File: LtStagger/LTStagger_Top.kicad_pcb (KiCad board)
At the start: 2 copper layers, 155 x 112 mm, 9 parts

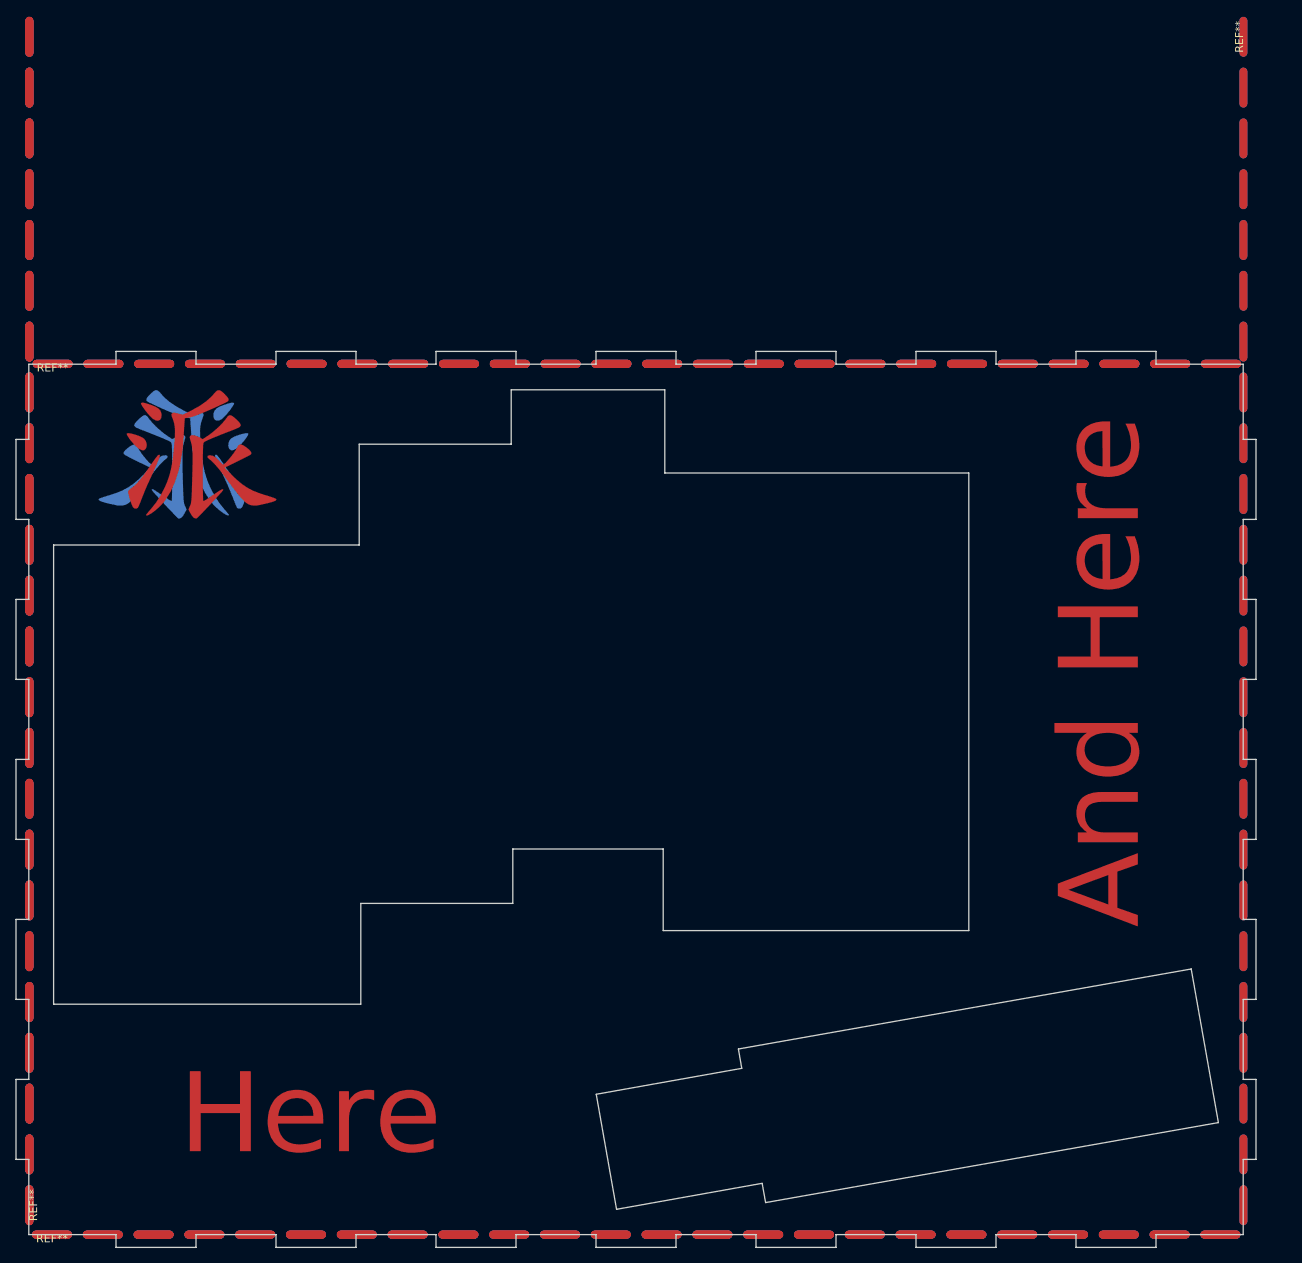
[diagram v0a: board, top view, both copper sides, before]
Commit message: about to give an angle and dog bones
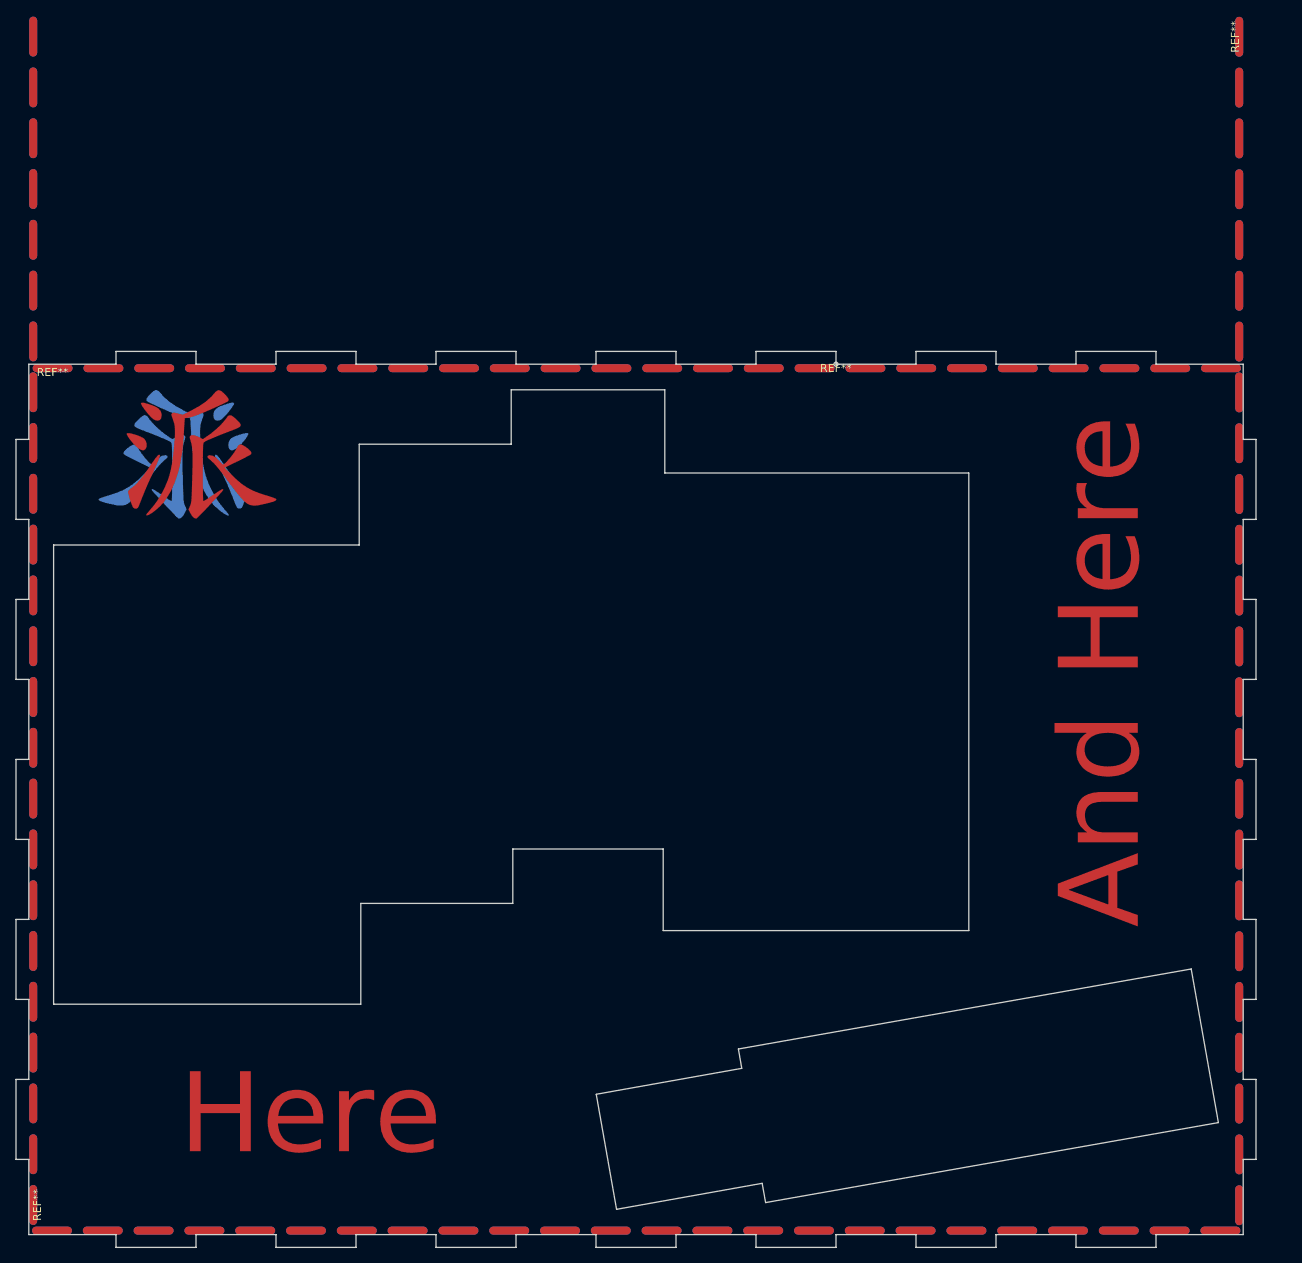
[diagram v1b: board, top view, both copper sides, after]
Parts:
- removed the REF** at (64.0, 147.5)
- removed the REF** at (66.8, 151.2)
- removed the REF** at (66.9, 42.4)
- added REF**: 0.5mmHole, Digi:0.5mmHole, F.Cu at (164.8, 42.4)
- moved REF** 0.55 mm to (66.9, 42.9)
- moved REF** 0.53 mm to (215.2, 1.48)
- moved REF** 0.50 mm to (66.8, 150.7)
- moved REF** 0.48 mm to (64.5, 147.5)

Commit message: Maybe ready for production
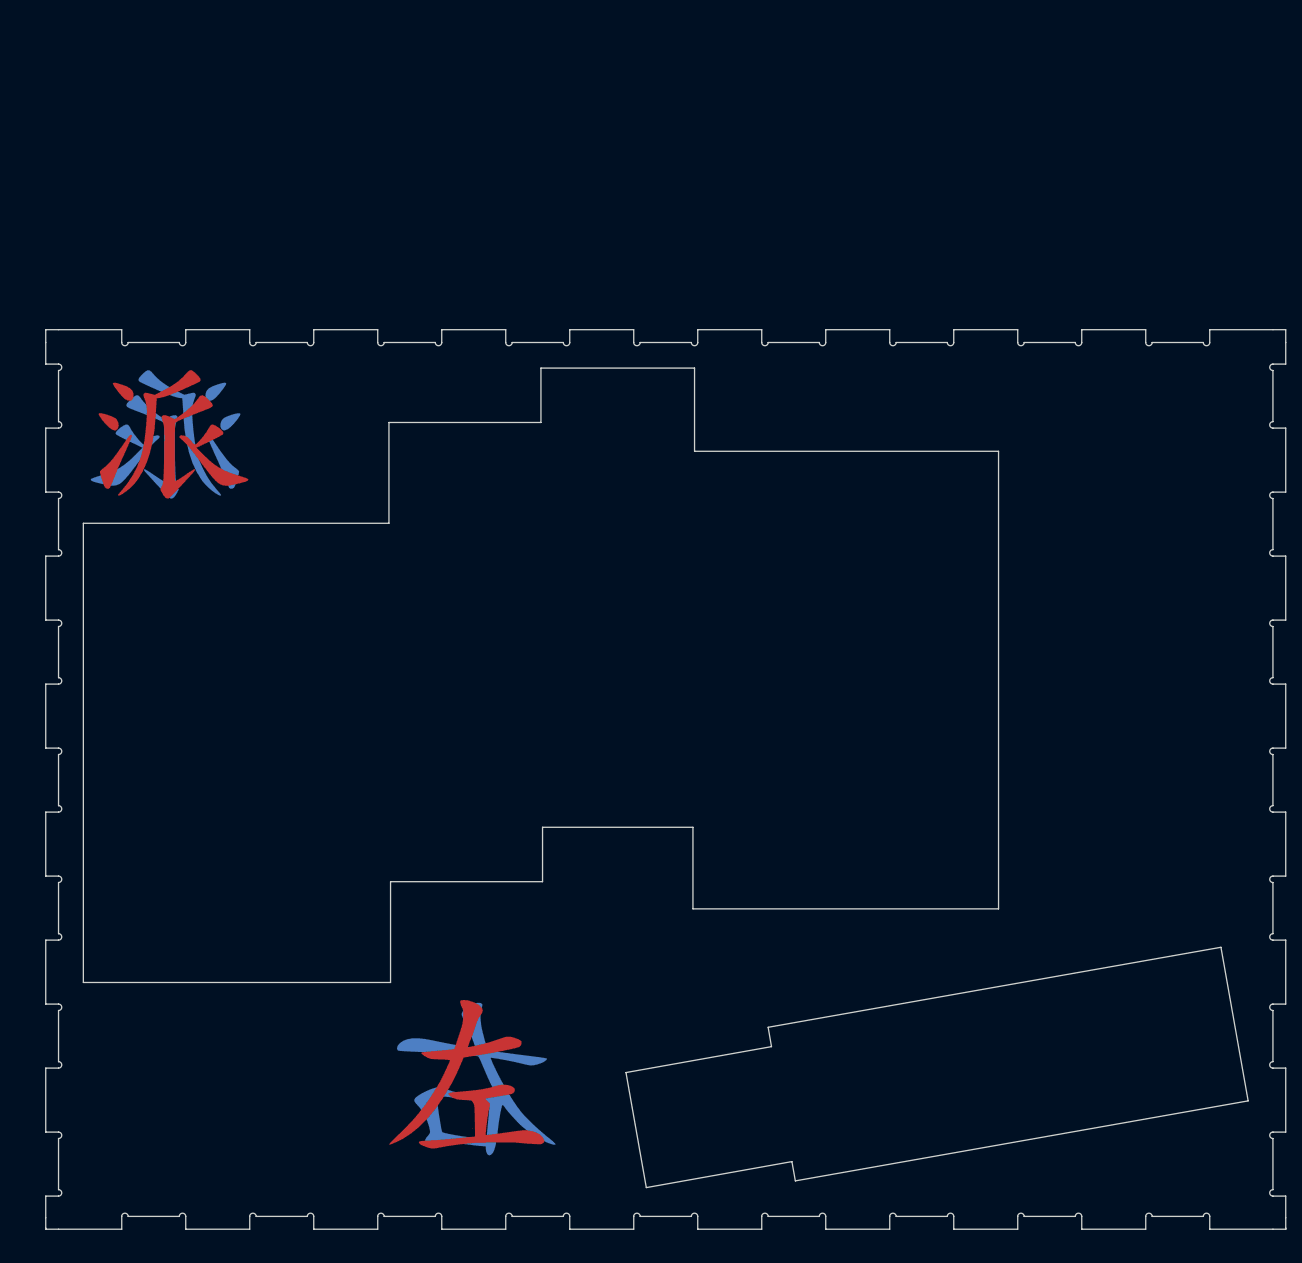
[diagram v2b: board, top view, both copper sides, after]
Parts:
- removed the G*** at (82.7, 53.5)
- removed the G*** at (84.8, 53.5)
- removed REF**: 0.5mmHole, Digi:0.5mmHole
- removed REF** (x4): Long pad, Digi:Long pad
- added ?: , Digi:Left, F.Cu at (119.4, 131.7)
- added ?: , Digi:Right, B.Cu at (119.4, 131.7)
- added G***: LOGO, Digi:PieCn, F.Cu at (81.3, 51.0)
- added G***: LOGO, Digi:PieCn, B.Cu at (81.7, 51.0)
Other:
- board size 155 x 112 mm -> 155 x 112.4 mm
- board text removed: "And Here"
- board text removed: "Here"
